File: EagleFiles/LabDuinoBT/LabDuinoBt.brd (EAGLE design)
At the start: 78.4 x 15.9 mm, 9 parts

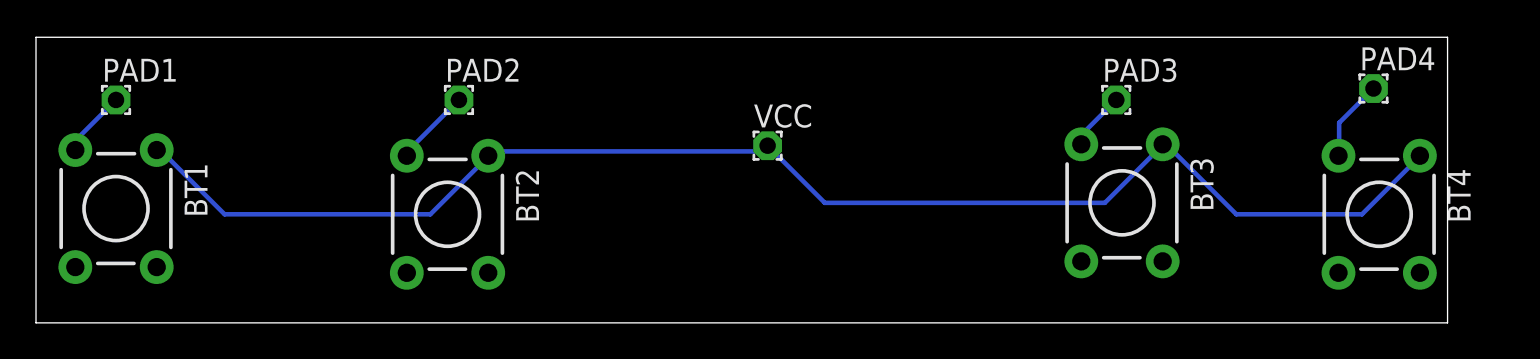
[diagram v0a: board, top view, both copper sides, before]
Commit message: Button Board UpDate
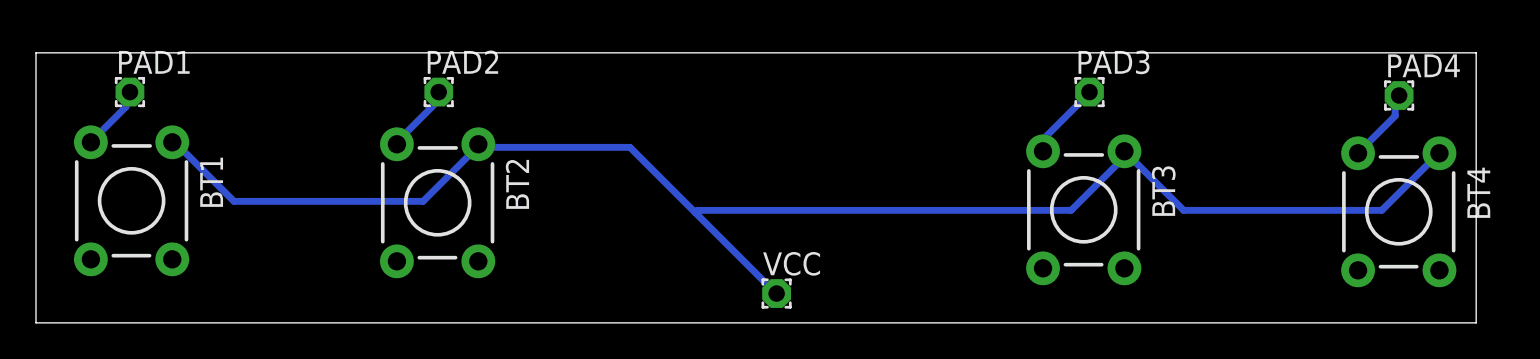
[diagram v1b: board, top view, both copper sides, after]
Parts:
- moved VCC 8.23 mm to (41.1, 1.63)
- moved BT3 2.16 mm to (58.2, 6.28)
- moved PAD3 1.55 mm to (58.5, 12.8)
- moved PAD4 1.48 mm to (75.7, 12.6)
- moved PAD2 1.21 mm to (22.4, 12.8)
- moved BT4 1.10 mm to (75.7, 6.17)
- moved BT1 0.97 mm to (5.31, 6.78)
- moved PAD1 0.89 mm to (5.22, 12.8)
- moved BT2 0.84 mm to (22.3, 6.67)
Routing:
- net VCC: track 78.8 -> 85.3 mm
- net N$3: track 3.51 -> 4.34 mm
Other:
- board size 78.4 x 15.9 mm -> 80 x 15 mm
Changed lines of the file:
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@@
 <setting verticaltext="up"/>
 </settings>
-<grid distance="0.0625" unitdist="inch" unit="inch" style="lines" multiple="1" display="no" altdistance="0.0625" altunitdist="inch" altunit="inch"/>
+<grid distance="0.5" unitdist="mm" unit="mm" style="lines" multiple="1" display="no" altdistance="0.5" altunitdist="mm" altunit="mm"/>
 <layers>
 <layer number="1" name="Top" color="4" fill="1" visible="yes" active="yes"/>
@@
 <board>
 <plain>
-<wire x1="0" y1="0" x2="78.41" y2="0" width="0" layer="20"/>
-<wire x1="78.41" y1="0" x2="78.41" y2="15.865" width="0" layer="20"/>
-<wire x1="78.41" y1="15.865" x2="0" y2="15.865" width="0" layer="20"/>
-<wire x1="0" y1="15.865" x2="0" y2="0" width="0" layer="20"/>
+<wire x1="0" y1="0" x2="80" y2="0" width="0" layer="20"/>
+<wire x1="80" y1="0" x2="80" y2="15" width="0" layer="20"/>
+<wire x1="80" y1="15" x2="0" y2="15" width="0" layer="20"/>
+<wire x1="0" y1="15" x2="0" y2="0" width="0" layer="20"/>
 </plain>
 <attributes>
@@
 </variantdefs>
 <classes>
-<class number="0" name="default" width="0" drill="0.508">
+<class number="0" name="default" width="0.381" drill="0.508">
 <clearance class="0" value="2"/>
 </class>
@@
 <description language="de">&lt;b&gt;EAGLE Design Rules&lt;/b&gt;
 &lt;p&gt;
-Die Standard-Design-Rules sind so gewÃ¤hlt, dass sie fÃ¼r
+Die Standard-Design-Rules sind so gewählt, dass sie für
 die meisten Anwendungen passen. Sollte ihre Platine
 besondere Anforderungen haben, treffen Sie die erforderlichen
@@
 <autorouter>
 <pass name="Default">
-<param name="RoutingGrid" value="12.5mil"/>
+<param name="RoutingGrid" value="50mil"/>
 <param name="AutoGrid" value="1"/>
 <param name="Efforts" value="0"/>
@@
 <param name="PrefDir.14" value="0"/>
 <param name="PrefDir.15" value="0"/>
-<param name="PrefDir.16" value="-"/>
+<param name="PrefDir.16" value="a"/>
 <param name="cfVia" value="8"/>
 <param name="cfNonPref" value="5"/>
@@
 </autorouter>
 <elements>
-<element name="BT1" library="SparkFun-Retired" package="TACTILE-PTH" value="" x="4.445" y="6.35" rot="R270"/>
-<element name="BT2" library="SparkFun-Retired" package="TACTILE-PTH" value="" x="22.86" y="6.0325" rot="R270"/>
-<element name="BT3" library="SparkFun-Retired" package="TACTILE-PTH" value="" x="60.325" y="6.6675" rot="R270"/>
-<element name="BT4" library="SparkFun-Retired" package="TACTILE-PTH" value="" x="74.6125" y="6.0325" rot="R270"/>
-<element name="PAD1" library="wirepad" package="1,6/0,9" value="" x="4.445" y="12.3825"/>
-<element name="PAD2" library="wirepad" package="1,6/0,9" value="" x="23.495" y="12.3825"/>
-<element name="PAD3" library="wirepad" package="1,6/0,9" value="" x="60.0075" y="12.3825"/>
-<element name="PAD4" library="wirepad" package="1,6/0,9" value="" x="74.295" y="13.0175"/>
-<element name="VCC" library="wirepad" package="1,6/0,9" value="" x="40.64" y="9.8425"/>
+<element name="BT1" library="SparkFun-Retired" package="TACTILE-PTH" value="" x="5.31" y="6.78" rot="R270"/>
+<element name="BT2" library="SparkFun-Retired" package="TACTILE-PTH" value="" x="22.31" y="6.67" rot="R270"/>
+<element name="BT3" library="SparkFun-Retired" package="TACTILE-PTH" value="" x="58.2" y="6.28" rot="R270"/>
+<element name="BT4" library="SparkFun-Retired" package="TACTILE-PTH" value="" x="75.7" y="6.17" rot="R270"/>
+<element name="PAD1" library="wirepad" package="1,6/0,9" value="" x="5.22" y="12.82"/>
+<element name="PAD2" library="wirepad" package="1,6/0,9" value="" x="22.37" y="12.82"/>
+<element name="PAD3" library="wirepad" package="1,6/0,9" value="" x="58.52" y="12.82"/>
+<element name="PAD4" library="wirepad" package="1,6/0,9" value="" x="75.72" y="12.63"/>
+<element name="VCC" library="wirepad" package="1,6/0,9" value="" x="41.14" y="1.63"/>
 </elements>
 <signals>
@@
 <contactref element="BT4" pad="1"/>
 <contactref element="VCC" pad="1"/>
-<wire x1="73.66" y1="6.0325" x2="76.835" y2="9.2075" width="0.254" layer="16"/>
-<wire x1="66.675" y1="6.0325" x2="73.66" y2="6.0325" width="0.254" layer="16"/>
-<wire x1="62.865" y1="9.8425" x2="66.675" y2="6.0325" width="0.254" layer="16"/>
-<wire x1="76.835" y1="9.2075" x2="76.8731" y2="9.2837" width="0.254" layer="16"/>
-<wire x1="62.865" y1="9.8425" x2="62.5856" y2="9.9187" width="0.254" layer="16"/>
-<wire x1="40.3225" y1="9.525" x2="40.64" y2="9.8425" width="0.254" layer="16"/>
-<wire x1="25.4" y1="9.525" x2="40.3225" y2="9.525" width="0.254" layer="16"/>
-<wire x1="25.4" y1="9.525" x2="25.1206" y2="9.2837" width="0.254" layer="16"/>
-<wire x1="10.4775" y1="6.0325" x2="6.985" y2="9.525" width="0.254" layer="16"/>
-<wire x1="21.9075" y1="6.0325" x2="10.4775" y2="6.0325" width="0.254" layer="16"/>
-<wire x1="25.0825" y1="9.2075" x2="21.9075" y2="6.0325" width="0.254" layer="16"/>
-<wire x1="6.985" y1="9.525" x2="6.7056" y2="9.6012" width="0.254" layer="16"/>
-<wire x1="25.0825" y1="9.2075" x2="25.1206" y2="9.2837" width="0.254" layer="16"/>
-<wire x1="59.3725" y1="6.6675" x2="62.5475" y2="9.8425" width="0.254" layer="16"/>
-<wire x1="43.815" y1="6.6675" x2="59.3725" y2="6.6675" width="0.254" layer="16"/>
-<wire x1="40.64" y1="9.8425" x2="43.815" y2="6.6675" width="0.254" layer="16"/>
-<wire x1="62.5475" y1="9.8425" x2="62.5856" y2="9.9187" width="0.254" layer="16"/>
+<wire x1="74.75" y1="6.25" x2="77.75" y2="9.25" width="0.381" layer="16"/>
+<wire x1="63.75" y1="6.25" x2="74.75" y2="6.25" width="0.381" layer="16"/>
+<wire x1="60.5" y1="9.5" x2="63.75" y2="6.25" width="0.381" layer="16"/>
+<wire x1="77.75" y1="9.25" x2="77.9606" y2="9.4212" width="0.381" layer="16"/>
+<wire x1="60.5" y1="9.5" x2="60.4606" y2="9.5312" width="0.381" layer="16"/>
+<wire x1="33" y1="9.75" x2="36.625" y2="6.125" width="0.381" layer="16"/>
+<wire x1="36.625" y1="6.125" x2="41" y2="1.75" width="0.381" layer="16"/>
+<wire x1="24.75" y1="9.75" x2="33" y2="9.75" width="0.381" layer="16"/>
+<wire x1="41" y1="1.75" x2="41.14" y2="1.63" width="0.381" layer="16"/>
+<wire x1="24.75" y1="9.75" x2="24.5706" y2="9.9212" width="0.381" layer="16"/>
+<wire x1="11" y1="6.75" x2="7.75" y2="10" width="0.381" layer="16"/>
+<wire x1="21.5" y1="6.75" x2="11" y2="6.75" width="0.381" layer="16"/>
+<wire x1="24.5" y1="9.75" x2="21.5" y2="6.75" width="0.381" layer="16"/>
+<wire x1="7.75" y1="10" x2="7.5706" y2="10.0312" width="0.381" layer="16"/>
+<wire x1="24.5" y1="9.75" x2="24.5706" y2="9.9212" width="0.381" layer="16"/>
+<wire x1="57.5" y1="6.25" x2="60.5" y2="9.25" width="0.381" layer="16"/>
+<wire x1="36.75" y1="6.25" x2="57.5" y2="6.25" width="0.381" layer="16"/>
+<wire x1="60.5" y1="9.25" x2="60.4606" y2="9.5312" width="0.381" layer="16"/>
+<wire x1="36.75" y1="6.25" x2="36.625" y2="6.125" width="0.381" layer="16"/>
 </signal>
 <signal name="N$1">
 <contactref element="BT1" pad="3"/>
 <contactref element="PAD1" pad="1"/>
-<wire x1="1.905" y1="9.8425" x2="4.445" y2="12.3825" width="0.254" layer="16"/>
-<wire x1="1.905" y1="9.8425" x2="2.1844" y2="9.6012" width="0.254" layer="16"/>
+<wire x1="5" y1="12" x2="5" y2="12.75" width="0.381" layer="16"/>
+<wire x1="3.25" y1="10.25" x2="5" y2="12" width="0.381" layer="16"/>
+<wire x1="5" y1="12.75" x2="5.22" y2="12.82" width="0.381" layer="16"/>
+<wire x1="3.25" y1="10.25" x2="3.0494" y2="10.0312" width="0.381" layer="16"/>
 </signal>
 <signal name="N$2">
 <contactref element="BT2" pad="3"/>
 <contactref element="PAD2" pad="1"/>
-<wire x1="20.6375" y1="9.525" x2="23.495" y2="12.3825" width="0.254" layer="16"/>
-<wire x1="20.6375" y1="9.525" x2="20.5994" y2="9.2837" width="0.254" layer="16"/>
+<wire x1="22.25" y1="12.25" x2="22.25" y2="12.75" width="0.381" layer="16"/>
+<wire x1="20" y1="10" x2="22.25" y2="12.25" width="0.381" layer="16"/>
+<wire x1="22.25" y1="12.75" x2="22.37" y2="12.82" width="0.381" layer="16"/>
+<wire x1="20" y1="10" x2="20.0494" y2="9.9212" width="0.381" layer="16"/>
 </signal>
 <signal name="N$3">
 <contactref element="BT3" pad="3"/>
 <contactref element="PAD3" pad="1"/>
-<wire x1="57.785" y1="10.16" x2="60.0075" y2="12.3825" width="0.254" layer="16"/>
-<wire x1="57.785" y1="10.16" x2="58.0644" y2="9.9187" width="0.254" layer="16"/>
+<wire x1="56" y1="10.25" x2="58.5" y2="12.75" width="0.381" layer="16"/>
+<wire x1="56" y1="9.75" x2="56" y2="10.25" width="0.381" layer="16"/>
+<wire x1="58.5" y1="12.75" x2="58.52" y2="12.82" width="0.381" layer="16"/>
+<wire x1="56" y1="9.75" x2="55.9394" y2="9.5312" width="0.381" layer="16"/>
 </signal>
 <signal name="N$4">
 <contactref element="BT4" pad="3"/>
 <contactref element="PAD4" pad="1"/>
-<wire x1="72.39" y1="11.1125" x2="74.295" y2="13.0175" width="0.254" layer="16"/>
-<wire x1="72.39" y1="9.525" x2="72.39" y2="11.1125" width="0.254" layer="16"/>
-<wire x1="72.39" y1="9.525" x2="72.3519" y2="9.2837" width="0.254" layer="16"/>
+<wire x1="75.5" y1="11.5" x2="75.5" y2="12.5" width="0.381" layer="16"/>
+<wire x1="73.5" y1="9.5" x2="75.5" y2="11.5" width="0.381" layer="16"/>
+<wire x1="75.5" y1="12.5" x2="75.72" y2="12.63" width="0.381" layer="16"/>
+<wire x1="73.5" y1="9.5" x2="73.4394" y2="9.4212" width="0.381" layer="16"/>
 </signal>
 </signals>
